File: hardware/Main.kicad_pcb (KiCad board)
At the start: 2 copper layers, 54.5 x 57.5 mm, 34 parts, among them Q1 DMG2305UX, SW1 Bourns PEC11R, SW2 Bourns PEC11R, U1 LM386, U2 RDA5807M_Module, U3 RPi_Pico_TH, U4 S-1206B50-M3T1U

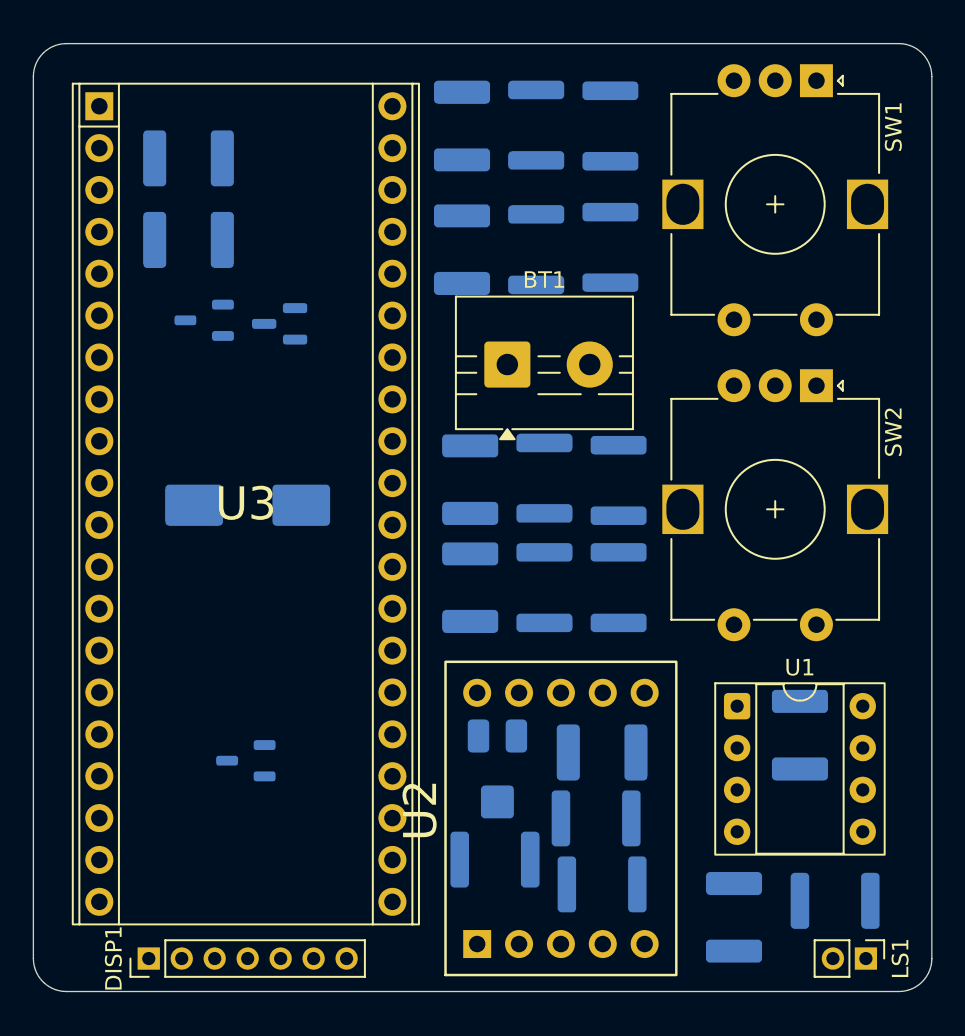
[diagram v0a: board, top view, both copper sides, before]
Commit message: Revised PCB Layout
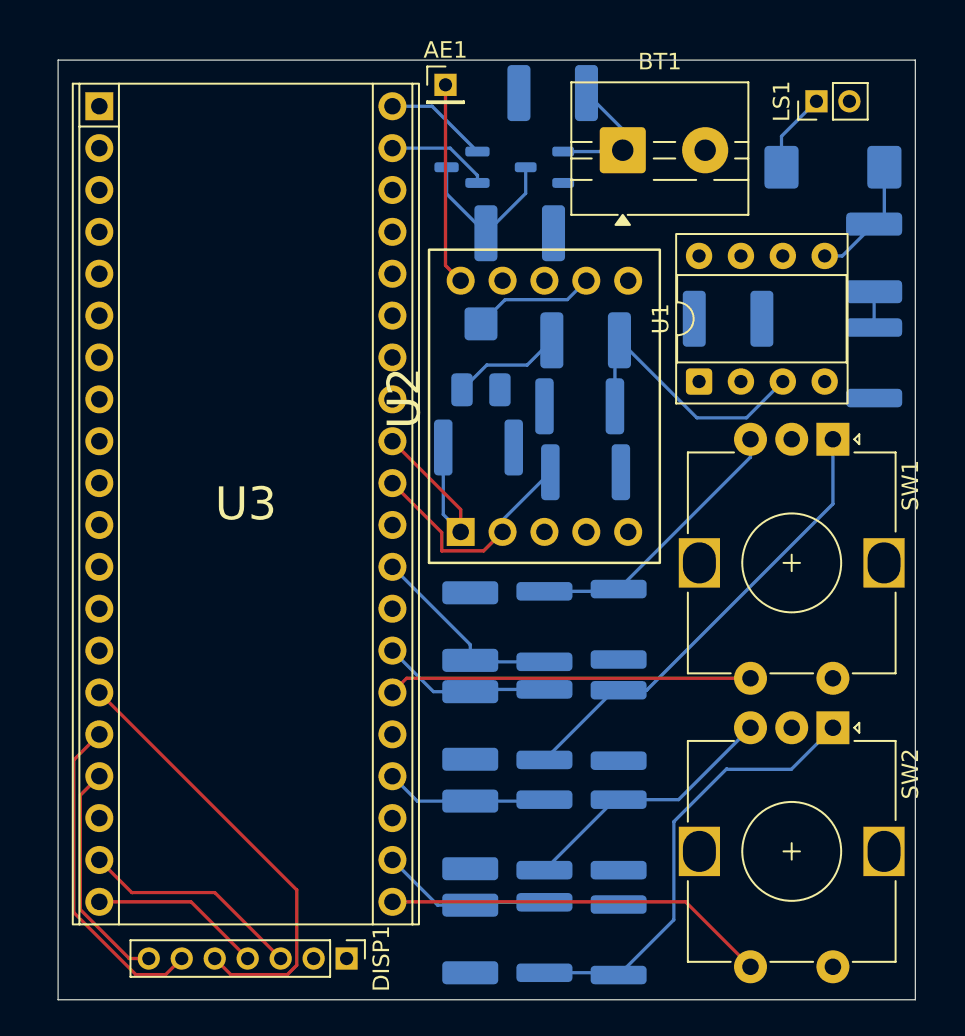
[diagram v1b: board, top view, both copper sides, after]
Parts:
- AE1: footprint Package_TO_SOT_SMD:SOT-23-3 -> Connector_PinHeader_2.00mm:PinHeader_1x01_P2.00mm_Vertical; moved to F.Cu
- C1: footprint Capacitor_SMD:CP_Elec_8x10 -> Capacitor_Tantalum_SMD:CP_EIA-7343-30_AVX-N
- RV1: value R_Potentiometer_Trim_US -> 10kΩ
- moved LS1 52.1 mm to (165.0, 72.0), turned to 90 degrees
- moved AE1 42.8 mm to (142.5, 71.0), turned to 0 degrees
- moved C1 41.0 mm to (166.0, 76.0)
- moved C2 40.9 mm to (168.5, 81.5)
- moved C8 36.4 mm to (144.0, 109.9)
- moved R10 36.4 mm to (148.5, 109.8)
- moved R12 36.4 mm to (153.0, 109.9)
- moved R1 32.7 mm to (168.5, 87.9), turned to -90 degrees
- moved C6 27.9 mm to (144.0, 122.8)
- moved R6 27.9 mm to (148.5, 122.7)
- moved R8 27.9 mm to (153.0, 122.9)
- moved C3 25.6 mm to (159.6, 85.2), turned to 0 degrees
- moved C4 25.0 mm to (151.0, 86.5)
- moved R2 25.0 mm to (150.6, 90.5)
- moved R3 25.0 mm to (144.5, 93.0)
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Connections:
- RV1 pad 1: Net-(C4-Pad1) -> GND
- RV1 pad 2: GND -> Net-(U2-ROUT)
- RV1 pad 3: Net-(U2-ROUT) -> Net-(C4-Pad1)
- U3 pad 1: /ENC2A -> unconnected-(U3-GP0-Pad1)
- U3 pad 10: /DISP_DC -> unconnected-(U3-GP7-Pad10)
- U3 pad 15: unconnected-(U3-GP11-Pad15) -> /DISP_RES
- U3 pad 16: unconnected-(U3-GP12-Pad16) -> /DISP_DC
- U3 pad 17: unconnected-(U3-GP13-Pad17) -> /DISP_CS
- U3 pad 19: /ENC1A -> /DISP_SCLK
- U3 pad 2: /ENC2B -> unconnected-(U3-GP1-Pad2)
- U3 pad 20: /ENC1B -> /DISP_SDA
- U3 pad 21: /Radio-Audio/Radio_SDA -> /ENC1_BTN
- U3 pad 22: /Radio-Audio/Radio_SCL -> /ENC1A
- U3 pad 24: unconnected-(U3-GP18-Pad24) -> /ENC1B
- U3 pad 26: unconnected-(U3-GP20-Pad26) -> /ENC2_BTN
- U3 pad 27: /ENC1_BTN -> /ENC2A
- U3 pad 29: /ENC2_BTN -> /ENC2B
- U3 pad 31: unconnected-(U3-GP26/ADC0-Pad31) -> /Radio-Audio/Radio_SCL
- U3 pad 32: unconnected-(U3-GP27/ADC1-Pad32) -> /Radio-Audio/Radio_SDA
- U3 pad 4: /DISP_SCLK -> unconnected-(U3-GP2-Pad4)
- U3 pad 5: /DISP_SDA -> unconnected-(U3-GP3-Pad5)
- U3 pad 7: /DISP_CS -> unconnected-(U3-GP5-Pad7)
- U3 pad 9: /DISP_RES -> unconnected-(U3-GP6-Pad9)
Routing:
- net Net-(R6-Pad2): track 0.00 -> 28.0 mm
- net Net-(R10-Pad2): track 0.00 -> 27.9 mm
- net /DISP_RES: track 0.00 -> 27.1 mm
- net /ENC1_BTN: track 0.00 -> 23.4 mm
- net /ENC2_BTN: track 0.00 -> 22.1 mm
- net /DISP_DC: track 0.00 -> 20.0 mm
- net Net-(R11-Pad1): track 0.00 -> 17.0 mm
- net Net-(U1-+): track 0.00 -> 16.9 mm
- net Net-(R5-Pad1): track 0.00 -> 16.1 mm
- net /Radio-Audio/Radio_SCL: track 0.00 -> 14.3 mm
- net /DISP_CS: track 0.00 -> 14.0 mm
- net /DISP_SCLK: track 0.00 -> 13.5 mm
- net /Radio-Audio/Radio_SDA: track 0.00 -> 12.8 mm
- net Net-(AE1-A): track 0.00 -> 12.3 mm
- net /ENC2B: track 0.00 -> 12.2 mm
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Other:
- board size 54.5 x 57.5 mm -> 52 x 57 mm
